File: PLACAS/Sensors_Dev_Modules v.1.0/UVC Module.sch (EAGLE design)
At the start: 12 parts, among them IC1 OPA4191ID

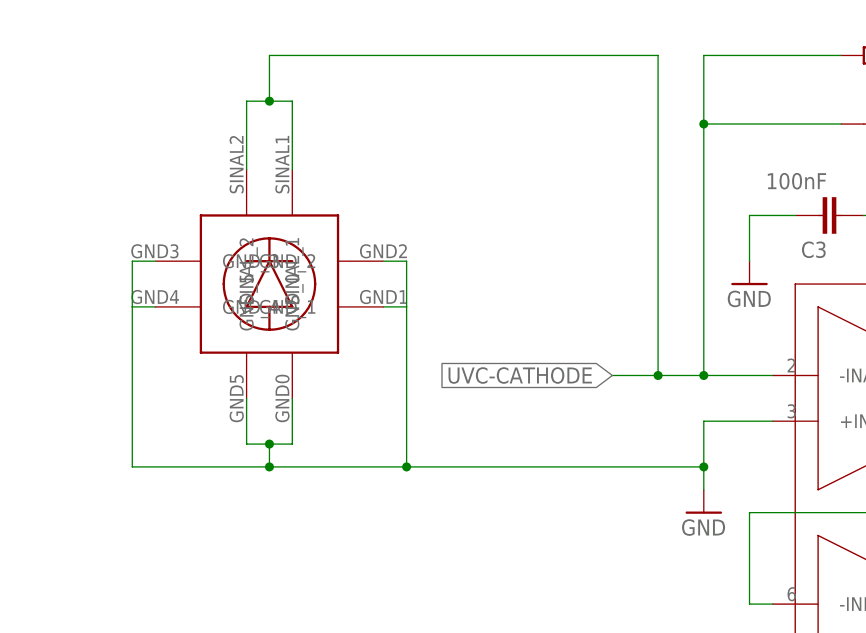
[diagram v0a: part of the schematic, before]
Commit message: Add files via upload
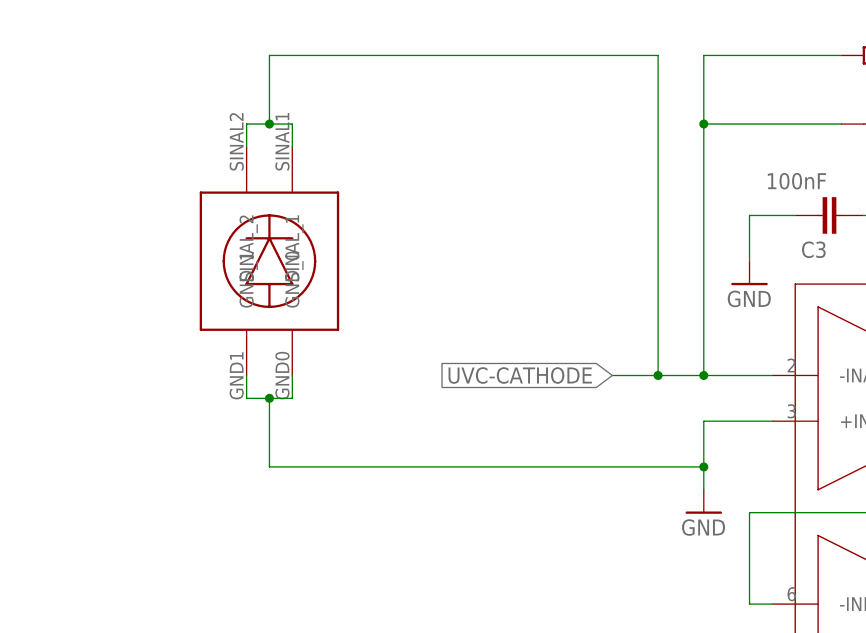
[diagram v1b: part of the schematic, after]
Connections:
- net GND: no longer U$1.GND_2, U$1.GND_3, U$1.GND_4, U$1.GND_5
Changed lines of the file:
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@@
 </classes>
 <parts>
-<part name="U$1" library="Zenith_Breakouts" deviceset="BREAKOUT_UV-C" device=""/>
 <part name="R2" library="rcl" library_urn="urn:adsk.eagle:library:334" deviceset="R-EU_" device="R0805" package3d_urn="urn:adsk.eagle:package:23553/2" value="18k"/>
 <part name="R3" library="rcl" library_urn="urn:adsk.eagle:library:334" deviceset="R-EU_" device="R0805" package3d_urn="urn:adsk.eagle:package:23553/2" value="10K"/>
@@
 <part name="P+2" library="supply1" library_urn="urn:adsk.eagle:library:371" deviceset="+5V" device=""/>
 <part name="P-2" library="supply1" library_urn="urn:adsk.eagle:library:371" deviceset="-5V" device=""/>
+<part name="U$1" library="Zenith_Breakouts" deviceset="BREAKOUT_UV-C" device=""/>
 </parts>
 <sheets>
@@
 </plain>
 <instances>
-<instance part="U$1" gate="G$1" x="10.16" y="119.38" smashed="yes" rot="R90"/>
 <instance part="R2" gate="G$1" x="101.6" y="68.58" smashed="yes">
 <attribute name="NAME" x="97.79" y="70.0786" size="1.778" layer="95"/>
@@
 <attribute name="VALUE" x="-2.54" y="71.12" size="1.778" layer="96" rot="R270"/>
 </instance>
+<instance part="U$1" gate="G$1" x="10.16" y="121.92" smashed="yes" rot="R90"/>
 </instances>
 <busses>
@@
 <wire x1="58.42" y1="104.14" x2="66.04" y2="104.14" width="0.1524" layer="91"/>
 <wire x1="58.42" y1="96.52" x2="58.42" y2="99.06" width="0.1524" layer="91"/>
+<wire x1="58.42" y1="99.06" x2="58.42" y2="104.14" width="0.1524" layer="91"/>
+<junction x="58.42" y="99.06"/>
+<pinref part="U$1" gate="G$1" pin="GND_1"/>
+<wire x1="10.16" y1="99.06" x2="58.42" y2="99.06" width="0.1524" layer="91"/>
+<wire x1="7.62" y1="109.22" x2="7.62" y2="106.68" width="0.1524" layer="91"/>
+<wire x1="7.62" y1="106.68" x2="10.16" y2="106.68" width="0.1524" layer="91"/>
 <pinref part="U$1" gate="G$1" pin="GND_0"/>
-<wire x1="58.42" y1="99.06" x2="58.42" y2="104.14" width="0.1524" layer="91"/>
-<wire x1="12.7" y1="101.6" x2="12.7" y2="106.68" width="0.1524" layer="91"/>
-<pinref part="U$1" gate="G$1" pin="GND_5"/>
-<wire x1="7.62" y1="106.68" x2="7.62" y2="101.6" width="0.1524" layer="91"/>
-<wire x1="7.62" y1="101.6" x2="10.16" y2="101.6" width="0.1524" layer="91"/>
-<wire x1="10.16" y1="101.6" x2="12.7" y2="101.6" width="0.1524" layer="91"/>
-<wire x1="10.16" y1="101.6" x2="10.16" y2="99.06" width="0.1524" layer="91"/>
-<junction x="10.16" y="101.6"/>
-<wire x1="10.16" y1="99.06" x2="25.4" y2="99.06" width="0.1524" layer="91"/>
-<junction x="58.42" y="99.06"/>
-<pinref part="U$1" gate="G$1" pin="GND_2"/>
-<wire x1="25.4" y1="99.06" x2="58.42" y2="99.06" width="0.1524" layer="91"/>
-<wire x1="22.86" y1="121.92" x2="25.4" y2="121.92" width="0.1524" layer="91"/>
-<pinref part="U$1" gate="G$1" pin="GND_1"/>
-<wire x1="25.4" y1="121.92" x2="25.4" y2="116.84" width="0.1524" layer="91"/>
-<wire x1="25.4" y1="116.84" x2="22.86" y2="116.84" width="0.1524" layer="91"/>
-<wire x1="25.4" y1="116.84" x2="25.4" y2="99.06" width="0.1524" layer="91"/>
-<junction x="25.4" y="99.06"/>
-<pinref part="U$1" gate="G$1" pin="GND_3"/>
-<wire x1="-2.54" y1="121.92" x2="-5.08" y2="121.92" width="0.1524" layer="91"/>
-<wire x1="-5.08" y1="121.92" x2="-5.08" y2="116.84" width="0.1524" layer="91"/>
-<pinref part="U$1" gate="G$1" pin="GND_4"/>
-<wire x1="-5.08" y1="116.84" x2="-2.54" y2="116.84" width="0.1524" layer="91"/>
-<wire x1="-5.08" y1="116.84" x2="-5.08" y2="99.06" width="0.1524" layer="91"/>
-<wire x1="-5.08" y1="99.06" x2="10.16" y2="99.06" width="0.1524" layer="91"/>
-<junction x="10.16" y="99.06"/>
+<wire x1="10.16" y1="106.68" x2="12.7" y2="106.68" width="0.1524" layer="91"/>
+<wire x1="12.7" y1="106.68" x2="12.7" y2="109.22" width="0.1524" layer="91"/>
+<wire x1="10.16" y1="106.68" x2="10.16" y2="99.06" width="0.1524" layer="91"/>
+<junction x="10.16" y="106.68"/>
 </segment>
 <segment>
@@
 <junction x="58.42" y="109.22"/>
 <pinref part="R4" gate="G$1" pin="1"/>
-<pinref part="U$1" gate="G$1" pin="SINAL_2"/>
-<wire x1="7.62" y1="132.08" x2="7.62" y2="139.7" width="0.1524" layer="91"/>
-<wire x1="7.62" y1="139.7" x2="10.16" y2="139.7" width="0.1524" layer="91"/>
-<pinref part="U$1" gate="G$1" pin="SINAL_1"/>
-<wire x1="10.16" y1="139.7" x2="12.7" y2="139.7" width="0.1524" layer="91"/>
-<wire x1="12.7" y1="139.7" x2="12.7" y2="132.08" width="0.1524" layer="91"/>
-<wire x1="10.16" y1="139.7" x2="10.16" y2="144.78" width="0.1524" layer="91"/>
-<junction x="10.16" y="139.7"/>
+<wire x1="10.16" y1="137.16" x2="10.16" y2="144.78" width="0.1524" layer="91"/>
 <wire x1="10.16" y1="144.78" x2="53.34" y2="144.78" width="0.1524" layer="91"/>
 <wire x1="53.34" y1="144.78" x2="53.34" y2="109.22" width="0.1524" layer="91"/>
 <junction x="53.34" y="109.22"/>
-</segment>
-</net>
+<pinref part="U$1" gate="G$1" pin="SINAL_2"/>
+<wire x1="7.62" y1="134.62" x2="7.62" y2="137.16" width="0.1524" layer="91"/>
+<wire x1="7.62" y1="137.16" x2="10.16" y2="137.16" width="0.1524" layer="91"/>
+<pinref part="U$1" gate="G$1" pin="SINAL_1"/>
+<wire x1="10.16" y1="137.16" x2="12.7" y2="137.16" width="0.1524" layer="91"/>
+<wire x1="12.7" y1="137.16" x2="12.7" y2="134.62" width="0.1524" layer="91"/>
+<junction x="10.16" y="137.16"/>
+</segment>
+</net>
